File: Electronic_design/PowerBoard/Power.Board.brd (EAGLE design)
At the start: 100 x 80 mm, 33 parts, among them IC1 788TV, IC2 788TV

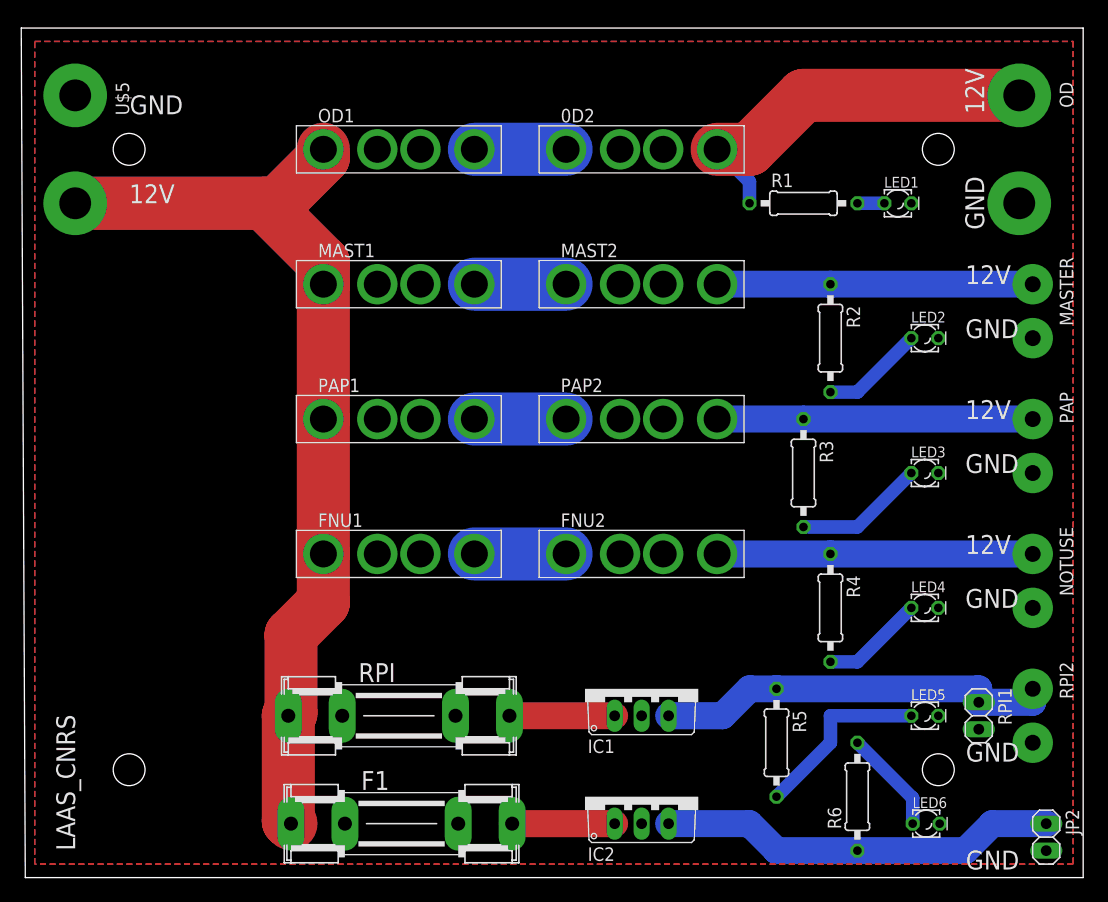
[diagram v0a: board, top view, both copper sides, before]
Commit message: ameliorations
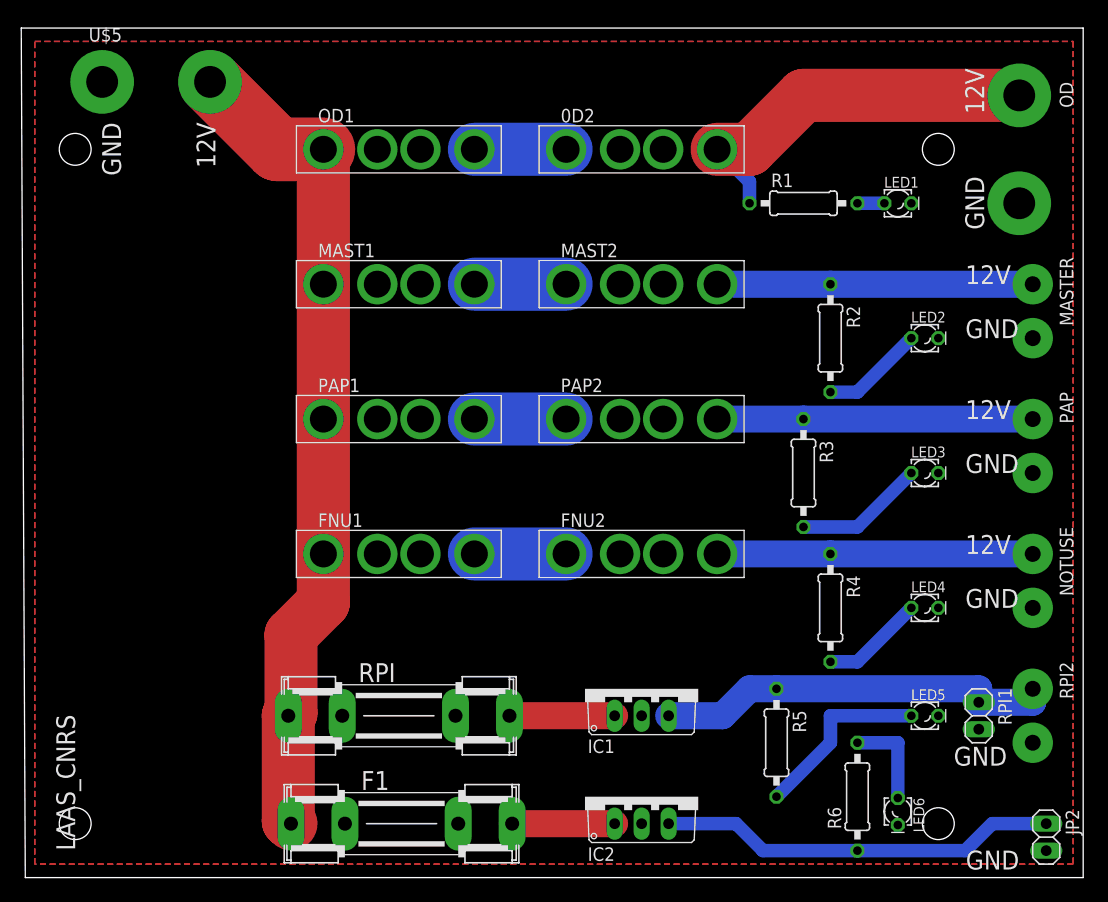
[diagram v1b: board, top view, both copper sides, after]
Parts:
- U$1: value TROU_FIXATION -> (none)
- moved LED6 2.90 mm to (82.5, 6.22), turned to 270 degrees
- moved U$5 2.84 mm to (7.62, 74.9), turned to 0 degrees
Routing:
- net 12V: track 124.0 -> 78.3 mm
- net N$17: track 9.78 -> 9.02 mm
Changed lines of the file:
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@@
 <wire x1="0" y1="80" x2="0.381" y2="0" width="0" layer="20"/>
 <text x="5.08" y="2.54" size="1.778" layer="25" font="vector" rot="R90">LAAS_CNRS</text>
-<text x="15.24" y="73.66" size="1.778" layer="25" font="vector" rot="R180">GND</text>
+<text x="7.62" y="71.12" size="1.778" layer="25" font="vector" rot="R270">GND</text>
 <text x="88.9" y="66.04" size="1.778" layer="25" font="vector" rot="R270">GND</text>
 <text x="88.9" y="50.8" size="1.778" layer="25" font="vector">GND</text>
@@
 <text x="88.9" y="25.4" size="1.778" layer="25" font="vector">GND</text>
 <text x="93.98" y="2.54" size="1.778" layer="25" font="vector" rot="R180">GND</text>
-<text x="93.98" y="12.7" size="1.778" layer="25" font="vector" rot="R180">GND</text>
-<text x="10.16" y="63.5" size="1.778" layer="25" font="vector">12V</text>
+<text x="92.837" y="12.319" size="1.778" layer="25" font="vector" rot="R180">GND</text>
+<text x="16.51" y="71.12" size="1.778" layer="25" font="vector" rot="R270">12V</text>
 <text x="88.9" y="76.2" size="1.778" layer="25" font="vector" rot="R270">12V</text>
 <text x="88.9" y="55.88" size="1.778" layer="25" font="vector">12V</text>
@@
 <element name="MAST1" library="AUTO_FUSE" package="AUTO_FUSE" value="AUTO_FUSE" x="35.56" y="55.88"/>
 <element name="PAP1" library="AUTO_FUSE" package="AUTO_FUSE" value="AUTO_FUSE" x="35.56" y="43.18"/>
-<element name="U$5" library="PowerHeaders" package="3MM_HEADER_2" value="3MM_HEADER_2" x="5.08" y="73.66" rot="R270"/>
+<element name="U$5" library="PowerHeaders" package="3MM_HEADER_2" value="3MM_HEADER_2" x="7.62" y="74.93"/>
 <element name="0D2" library="AUTO_FUSE" package="AUTO_FUSE" value="AUTO_FUSE" x="58.42" y="68.58"/>
 <element name="MAST2" library="AUTO_FUSE" package="AUTO_FUSE" value="AUTO_FUSE" x="58.42" y="55.88"/>
@@
 <attribute name="SPICEPREFIX" value="R" x="78.74" y="7.62" size="1.778" layer="27" rot="R90" display="off"/>
 </element>
-<element name="LED6" library="eagle-ltspice" library_urn="urn:adsk.eagle:library:217" package="LED_LD260" package3d_urn="urn:adsk.eagle:package:13313/1" value="" x="85.217" y="5.08">
-<attribute name="SPICEMODEL" value="NONE" x="85.217" y="5.08" size="1.778" layer="27" display="off"/>
-<attribute name="SPICEPREFIX" value="D" x="85.217" y="5.08" size="1.778" layer="27" display="off"/>
-<attribute name="SPICETYPE" value="diode" x="85.217" y="5.08" size="1.778" layer="27" display="off"/>
+<element name="LED6" library="eagle-ltspice" library_urn="urn:adsk.eagle:library:217" package="LED_LD260" package3d_urn="urn:adsk.eagle:package:13313/1" value="" x="82.55" y="6.223" rot="R270">
+<attribute name="SPICEMODEL" value="NONE" x="82.55" y="6.223" size="1.778" layer="27" rot="R270" display="off"/>
+<attribute name="SPICEPREFIX" value="D" x="82.55" y="6.223" size="1.778" layer="27" rot="R270" display="off"/>
+<attribute name="SPICETYPE" value="diode" x="82.55" y="6.223" size="1.778" layer="27" rot="R270" display="off"/>
 </element>
 <element name="IC2" library="linear" library_urn="urn:adsk.eagle:library:262" package="TO220V" package3d_urn="urn:adsk.eagle:package:16417/1" value="788TV" x="58.42" y="7.62"/>
-<element name="U$1" library="Trous_fixation" package="TROUS_FIXATION" value="TROU_FIXATION" x="0" y="0"/>
+<element name="U$1" library="Trous_fixation" package="TROUS_FIXATION" value="" x="0" y="0"/>
 </elements>
 <signals>
@@
 <contactref element="RPI" pad="1A"/>
 <contactref element="FNU1" pad="P$2"/>
-<wire x1="22.86" y1="63.5" x2="5.08" y2="63.5" width="5" layer="16"/>
-<wire x1="22.86" y1="63.5" x2="24.13" y2="63.5" width="5" layer="16"/>
-<wire x1="24.13" y1="63.5" x2="28.45" y2="67.82" width="5" layer="16"/>
-<wire x1="28.45" y1="67.82" x2="28.45" y2="68.58" width="5" layer="16"/>
-<wire x1="28.45" y1="57.91" x2="28.45" y2="55.88" width="5" layer="16"/>
-<wire x1="28.45" y1="57.91" x2="22.86" y2="63.5" width="5" layer="16"/>
-<wire x1="28.45" y1="67.82" x2="28.45" y2="68.58" width="5" layer="1"/>
-<wire x1="22.86" y1="63.5" x2="24.13" y2="63.5" width="5" layer="1"/>
-<wire x1="24.13" y1="63.5" x2="28.45" y2="67.82" width="5" layer="1"/>
-<wire x1="28.45" y1="57.91" x2="28.45" y2="55.88" width="5" layer="1"/>
-<wire x1="28.45" y1="57.91" x2="22.86" y2="63.5" width="5" layer="1"/>
 <wire x1="28.45" y1="55.88" x2="28.45" y2="43.18" width="5" layer="1"/>
 <wire x1="28.45" y1="43.18" x2="28.45" y2="30.48" width="5" layer="1"/>
@@
 <wire x1="25.146" y1="15.24" x2="25.146" y2="5.334" width="5" layer="1"/>
 <wire x1="25.146" y1="5.334" x2="25.4" y2="5.08" width="5" layer="1"/>
-<wire x1="5.08" y1="63.5" x2="22.86" y2="63.5" width="5" layer="1"/>
+<wire x1="28.45" y1="68.58" x2="28.45" y2="55.88" width="5" layer="1"/>
+<wire x1="17.78" y1="74.93" x2="24.13" y2="68.58" width="6" layer="1"/>
+<wire x1="24.13" y1="68.58" x2="28.45" y2="68.58" width="6" layer="1"/>
 </signal>
 <signal name="N$2">
@@
 <contactref element="R6" pad="1"/>
 <contactref element="IC2" pad="3"/>
-<wire x1="60.96" y1="5.08" x2="68.58" y2="5.08" width="2.54" layer="16"/>
-<wire x1="68.58" y1="5.08" x2="71.12" y2="2.54" width="2.54" layer="16"/>
-<wire x1="71.12" y1="2.54" x2="78.74" y2="2.54" width="2.54" layer="16"/>
-<wire x1="78.74" y1="2.54" x2="88.9" y2="2.54" width="2.54" layer="16"/>
-<wire x1="88.9" y1="2.54" x2="91.44" y2="5.08" width="2.54" layer="16"/>
-<wire x1="91.44" y1="5.08" x2="96.52" y2="5.08" width="2.54" layer="16"/>
+<wire x1="60.96" y1="5.08" x2="67.31" y2="5.08" width="1.27" layer="16"/>
+<wire x1="67.31" y1="5.08" x2="69.85" y2="2.54" width="1.27" layer="16"/>
+<wire x1="69.85" y1="2.54" x2="78.74" y2="2.54" width="1.27" layer="16"/>
+<wire x1="78.74" y1="2.54" x2="88.9" y2="2.54" width="1.27" layer="16"/>
+<wire x1="88.9" y1="2.54" x2="91.44" y2="5.08" width="1.27" layer="16"/>
+<wire x1="91.44" y1="5.08" x2="96.52" y2="5.08" width="1.27" layer="16"/>
 </signal>
 <signal name="N$5">
@@
 <contactref element="R6" pad="2"/>
 <contactref element="LED6" pad="A"/>
-<wire x1="78.74" y1="12.7" x2="83.947" y2="7.493" width="1.27" layer="16"/>
-<wire x1="83.947" y1="7.493" x2="83.947" y2="5.08" width="1.27" layer="16"/>
+<wire x1="78.74" y1="12.7" x2="82.55" y2="12.7" width="1.27" layer="16"/>
+<wire x1="82.55" y1="12.7" x2="82.55" y2="7.493" width="1.27" layer="16"/>
 </signal>
 <signal name="N$18">
